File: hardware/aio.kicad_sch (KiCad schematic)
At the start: 48 parts, among them Q1 FCX690BTA, Q2 NTF2955T1G, Q3 MMBT2907ALT1G, U1 XTR117AIDGKR, U10 REF3040AIDBZR, U11 KF301-5.0-2P, U12 TLV9301IDBVR, U2 ISO7041FDBQR, U23 KF301-5.0-2P, U28 DAC8551IADGKR, U4 DAC60501MDGSR, U5 XTR111AIDGQR, U6 TLV9301IDBVR, U7 INA226AIDGSR, U8 DAC60501MDGSR, U9 DAC60501MDGSR

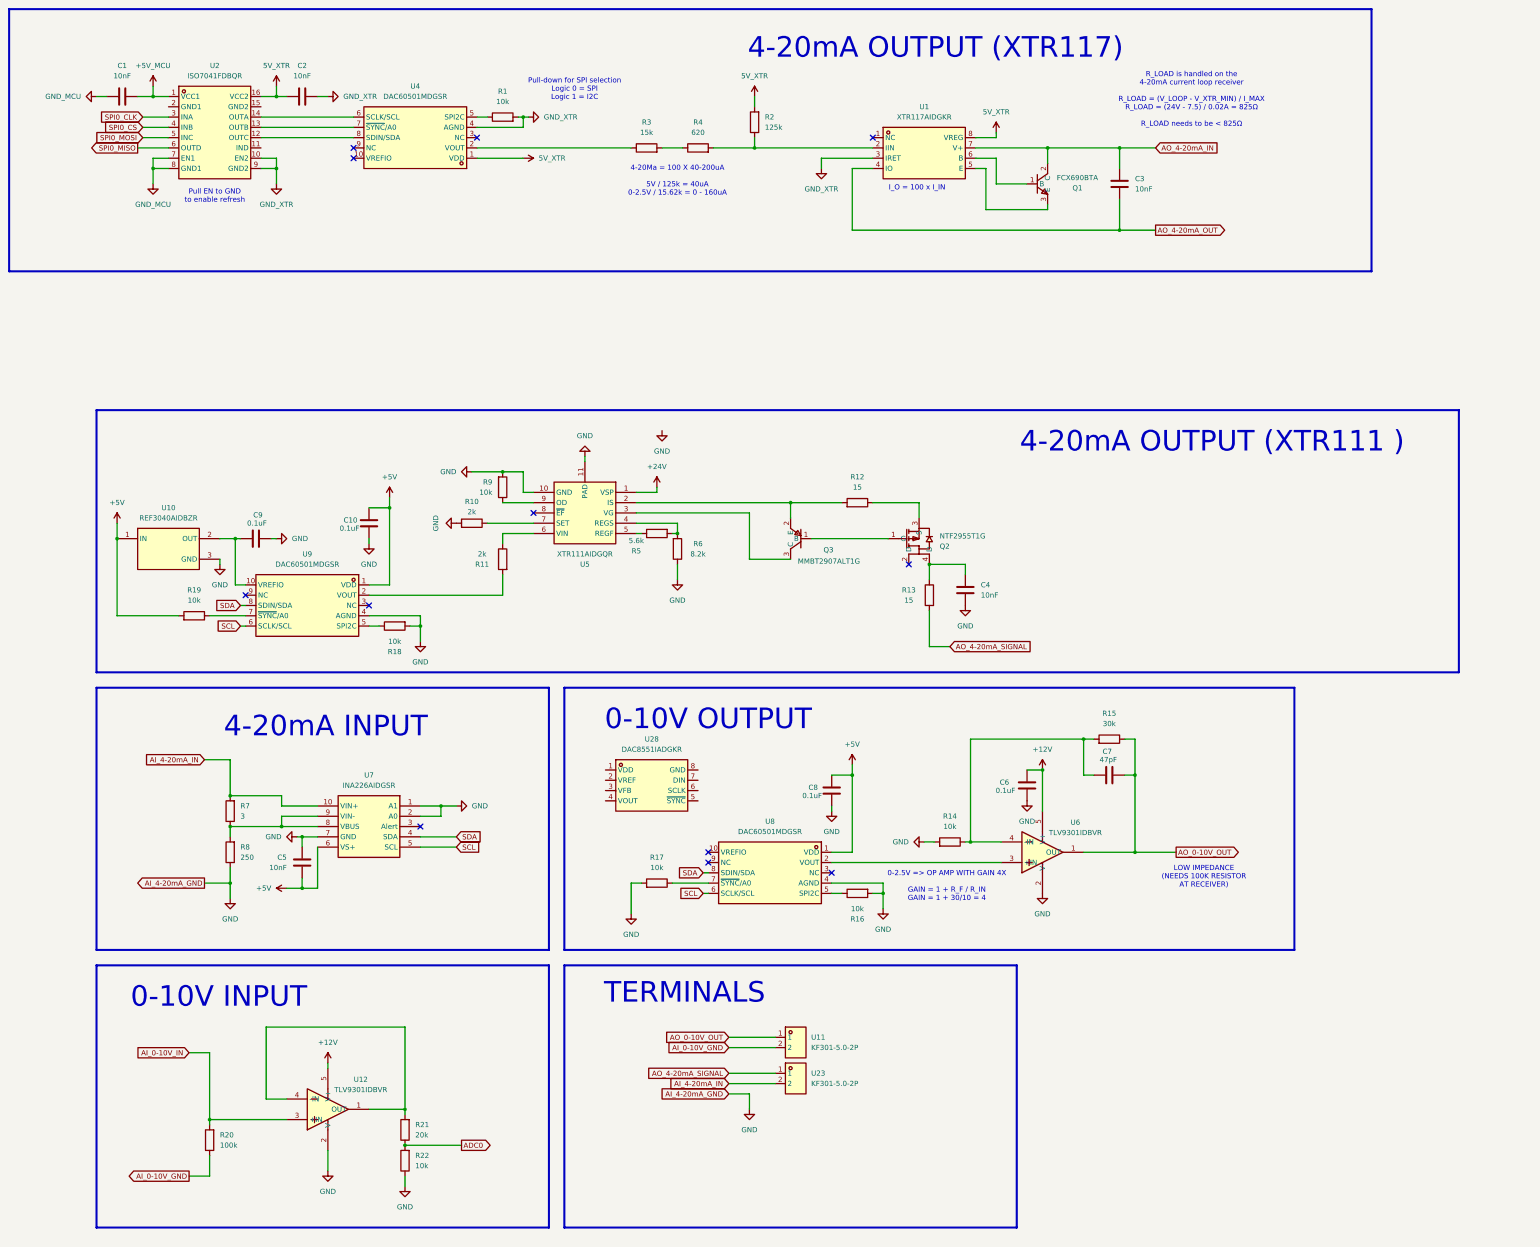
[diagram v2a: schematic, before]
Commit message: Board complete
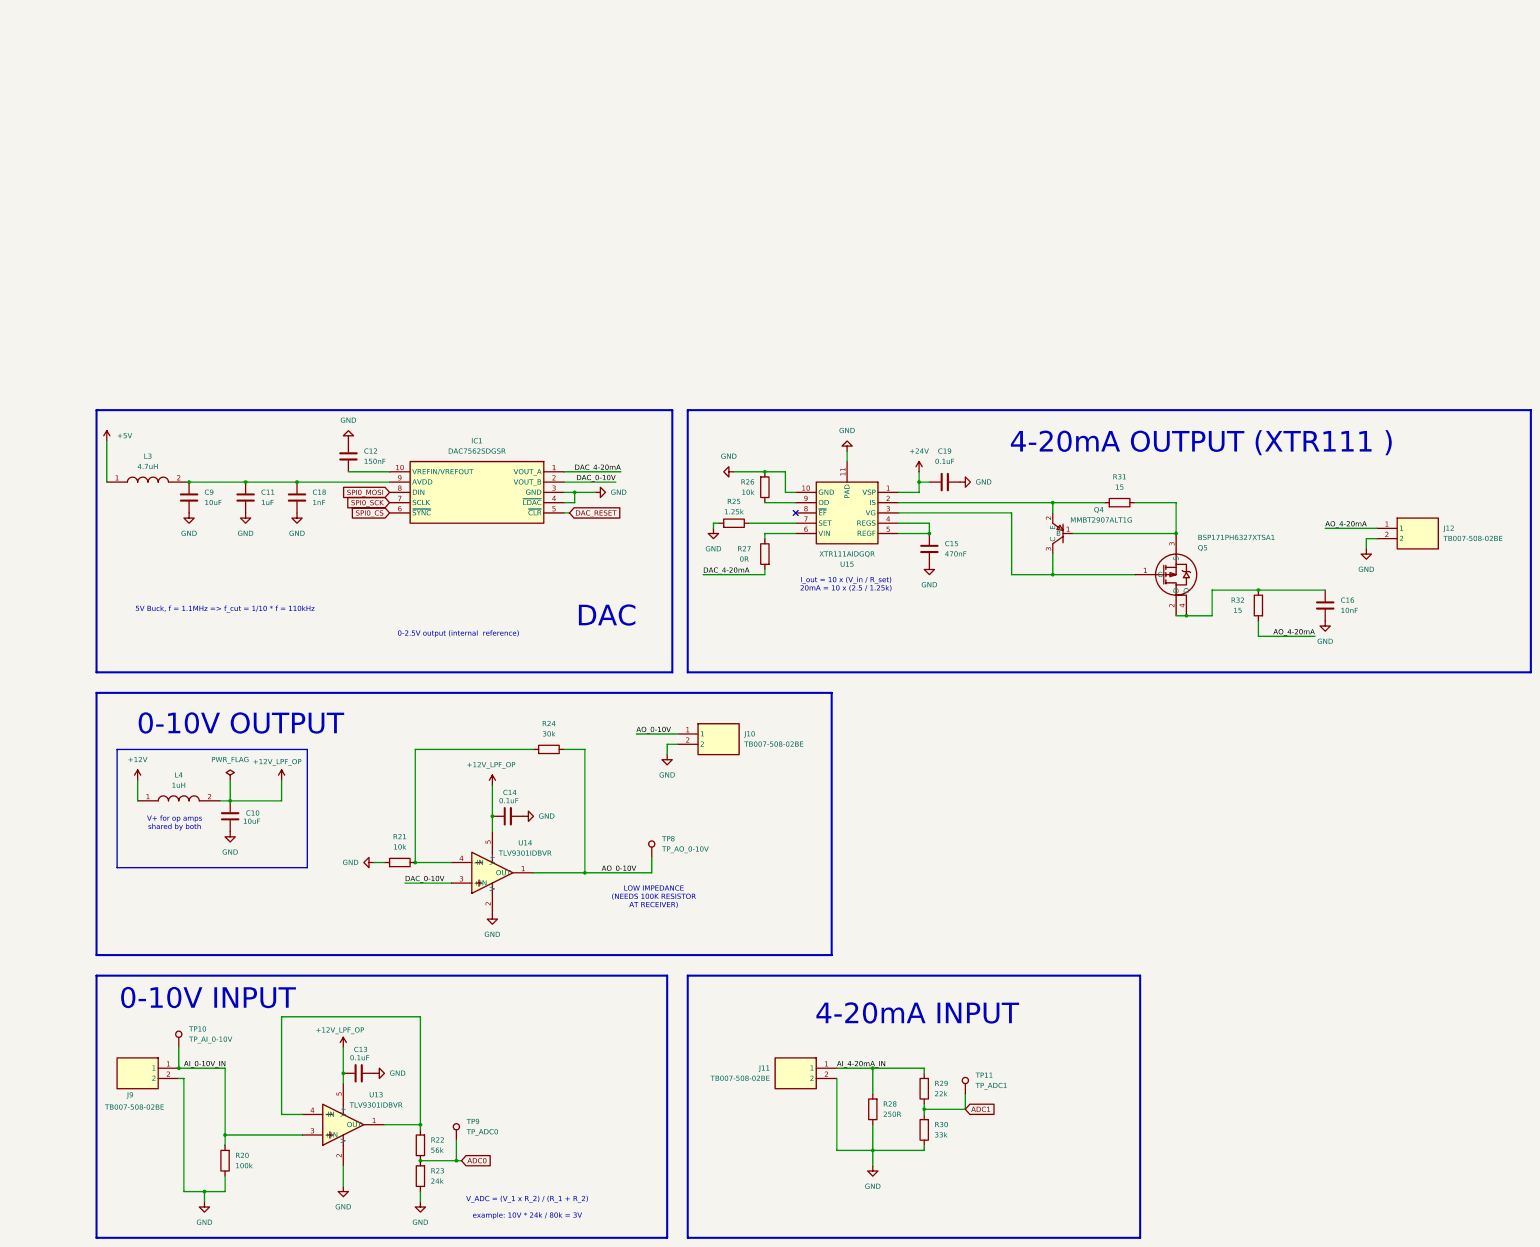
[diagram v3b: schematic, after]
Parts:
- removed C1, C2, C3, C5: 10nF, symbol Device:C
- removed C6, C8: 0.1uF, symbol Device:C
- removed C7: 47pF, symbol Device:C
- removed Q1: FCX690BTA, EasyEDA:SOT-89-3_L4.5-W2.5-P1.50-LS4.2-BR, symbol EasyEDA:FCX690BTA
- removed Q2: NTF2955T1G, EasyEDA:SOT-223-4_L6.5-W3.5-P2.30-LS7.0-BR, symbol EasyEDA:NTF2955T1G
- removed R1, R16, R17, R18, R19: 10k, symbol Device:R
- removed R2: 125k, symbol Device:R
- removed R3: 15k, symbol Device:R
- removed R4: 620, symbol Device:R
- removed R5: 5.6k, symbol Device:R
- removed R6: 8.2k, symbol Device:R
- removed R7: 3, symbol Device:R
- removed U1: XTR117AIDGKR, EasyEDA:VSSOP-8_L3.0-W3.0-P0.65-LS5.0-BL, symbol EasyEDA:XTR117AIDGKR
- removed U10: REF3040AIDBZR, EasyEDA:SOT-23-3_L2.9-W1.6-P1.90-LS2.8-BR, symbol EasyEDA:REF3040AIDBZR
- removed U11, U23: KF301-5.0-2P, EasyEDA:CONN-TH_P5.00_KF301-5.0-2P, symbol EasyEDA:KF301-5.0-2P
- removed U2: ISO7041FDBQR, EasyEDA:SSOP-16_L4.9-W3.9-P0.64-LS6.0-BL, symbol EasyEDA:ISO7041FDBQR
- removed U28: DAC8551IADGKR, EasyEDA:VSSOP-8_L3.0-W3.0-P0.65-LS5.0-BL, symbol EasyEDA:DAC8551IADGKR
- removed U4, U8, U9: DAC60501MDGSR, EasyEDA:VSSOP-10_L3.0-W3.0-P0.50-LS4.9-BL, symbol EasyEDA:DAC60501MDGSR
- removed U7: INA226AIDGSR, EasyEDA:MSOP-10_L3.0-W3.0-P0.50-LS5.0-BL, symbol EasyEDA:INA226AIDGSR
- added C11: 1uF, Capacitor_SMD:C_1206_3216Metric_Pad1.33x1.80mm_HandSolder, symbol Device:C
- added C12: 150nF, Capacitor_SMD:C_1206_3216Metric_Pad1.33x1.80mm_HandSolder, symbol Device:C
- added C13, C14, C19: 0.1uF, Capacitor_SMD:C_1206_3216Metric_Pad1.33x1.80mm_HandSolder, symbol Device:C
- added C15: 470nF, Capacitor_SMD:C_1206_3216Metric_Pad1.33x1.80mm_HandSolder, symbol Device:C
- added C18: 1nF, Capacitor_SMD:C_1206_3216Metric_Pad1.33x1.80mm_HandSolder, symbol Device:C
- added IC1: DAC7562SDGSR, Samacsys:SOP50P490X110-10N, symbol Samacsys:DAC7562SDGSR
- added J10, J11, J12, J9: TB007-508-02BE, Samacsys:TB00750802BE, symbol Samacsys:TB007-508-02BE
- added L3: 4.7uH, Samacsys:INDC3225X120N, symbol Samacsys:LQM31PN4R7M00L
- added L4: 1uH, Samacsys:LQM31PN1R0M00L, symbol Samacsys:LQM31PN1R0M00L
- added Q5: BSP171PH6327XTSA1, EasyEDA:SOT-223-4_L6.5-W3.5-P2.30-LS7.0-BR, symbol EasyEDA:BSP171PH6327XTSA1
- added R29: 22k, Resistor_SMD:R_1206_3216Metric_Pad1.30x1.75mm_HandSolder, symbol Device:R
- added R30: 33k, Resistor_SMD:R_1206_3216Metric_Pad1.30x1.75mm_HandSolder, symbol Device:R
- added TP10: TP_AI_0-10V, TestPoint:TestPoint_THTPad_2.0x2.0mm_Drill1.0mm, symbol Connector:TestPoint
- added TP11: TP_ADC1, TestPoint:TestPoint_THTPad_2.0x2.0mm_Drill1.0mm, symbol Connector:TestPoint
- added TP8: TP_AO_0-10V, TestPoint:TestPoint_THTPad_2.0x2.0mm_Drill1.0mm, symbol Connector:TestPoint
- added TP9: TP_ADC0, TestPoint:TestPoint_THTPad_2.0x2.0mm_Drill1.0mm, symbol Connector:TestPoint
- C10, C9: value 0.1uF -> 10uF; footprint (none) -> Capacitor_SMD:C_1206_3216Metric_Pad1.33x1.80mm_HandSolder
- C16: renamed from C4; footprint (none) -> Capacitor_SMD:C_1206_3216Metric_Pad1.33x1.80mm_HandSolder
- R20: footprint (none) -> Resistor_SMD:R_1206_3216Metric_Pad1.30x1.75mm_HandSolder
- R21: renamed from R14; footprint (none) -> Resistor_SMD:R_1206_3216Metric_Pad1.30x1.75mm_HandSolder
- R22: renamed from R21; value 20k -> 56k; footprint (none) -> Resistor_SMD:R_1206_3216Metric_Pad1.30x1.75mm_HandSolder
- R23: renamed from R22; value 10k -> 24k; footprint (none) -> Resistor_SMD:R_1206_3216Metric_Pad1.30x1.75mm_HandSolder
- R24: renamed from R15; footprint (none) -> Resistor_SMD:R_1206_3216Metric_Pad1.30x1.75mm_HandSolder
- R25: renamed from R10; value 2k -> 1.25k; footprint (none) -> Resistor_SMD:R_1206_3216Metric_Pad1.30x1.75mm_HandSolder
- R26: renamed from R9; footprint (none) -> Resistor_SMD:R_1206_3216Metric_Pad1.30x1.75mm_HandSolder
- R27: renamed from R11; value 2k -> 0R; footprint (none) -> Resistor_SMD:R_1206_3216Metric_Pad1.30x1.75mm_HandSolder
- R28: renamed from R8; value 250 -> 250R; footprint (none) -> Resistor_SMD:R_1206_3216Metric_Pad1.30x1.75mm_HandSolder
- R31: renamed from R12; footprint (none) -> Resistor_SMD:R_1206_3216Metric_Pad1.30x1.75mm_HandSolder
- R32: renamed from R13; footprint (none) -> Resistor_SMD:R_1206_3216Metric_Pad1.30x1.75mm_HandSolder
- renumbered Q3 to Q4, U12 to U13, U6 to U14, U5 to U15
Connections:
- net AI_0-10V_GND is gone; now on net GND: R20.1
- net +12V: now also L4.1; no longer U13.5 (V+), U14.5 (V+)
- net +24V: now also C19.2
- net +5V: now also L3.1; no longer C10.2
- net ADC0: now also TP9.1
- net AI_0-10V_IN: now also J9.1, TP10.1
- net AI_4-20mA_IN: now also R28.2, J11.1, R29.2
- net GND: now also C10.2, C11.1, C12.2, C13.2, C14.2, C15.1, C18.1, C19.1, IC1.3 (GND), IC1.4 (~{LDAC}), J10.2, J11.2, J12.2, J9.2, R30.1; no longer C10.1
- net SPI0_CS: now also IC1.6 (~{SYNC})
- net SPI0_MOSI: now also IC1.8 (DIN)
- net at Q4.1 (B): now also R31.1, Q5.3 (S)
- net at Q4.3 (C), U15.3 (VG): now also Q5.1 (G)
- net DAC_0-10V: now reaches U14.3 (+IN)
- net DAC_0-10V: now also IC1.2 (VOUT_B)
- net at U15.5 (REGF): now also U15.4 (REGS), C15.2
- net DAC_4-20mA: now reaches R27.2
- net DAC_4-20mA: now also IC1.1 (VOUT_A)
- net at C16.2, R32.1: now also Q5.2 (D), Q5.4 (D)
- net at C9.1: now also C11.2, C18.2, IC1.9 (AVDD), L3.2
- net AO_0-10V_OUT renamed AO_0-10V
- net AO_0-10V: now also J10.1, TP8.1
- net AO_4-20mA_SIGNAL renamed AO_4-20mA
- net AO_4-20mA: now also J12.1
- new net: C12.1, IC1.10 (VREFIN/VREFOUT)
- new net +12V_LPF_OP: C10.1, C13.1, C14.1, L4.2, U13.5 (V+), U14.5 (V+)
- new net ADC1: R29.1, R30.2, TP11.1
- new net DAC_RESET: IC1.5 (~{CLR})
- new net SPI0_SCK: IC1.7 (SCLK)
- no-connect marks 12 -> 1
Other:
- note added: "0-2.5V output (internal reference)"
- note added: "5V Buck, f = 1.1MHz => f_cut = 1/10 * f = 110kHz"
- note added: "DAC"
- note added: "I_out = 10 x (V_in / R_set) 20mA = 10 x (2.5 / 1.25k)"
- note added: "V+ for op amps shared by both"
- note added: "V_ADC = (V_1 x R_2) / (R_1 + R_2) example: 10V * 24k / 80k = 3V"
- note removed: "0-2.5V => OP AMP WITH GAIN 4X GAIN = 1 + R_F / R_IN GAIN = 1 + 30/10 = 4"
- note removed: "4-20Ma = 100 X 40-200uA 5V / 125k = 40uA 0-2.5V / 15.62k = 0 - 160uA"
- note removed: "4-20mA OUTPUT (XTR117)"
- note removed: "I_O = 100 x I_IN"
- note removed: "Pull EN to GND to enable refresh"
- note removed: "Pull-down for SPI selection Logic 0 = SPI Logic 1 = I2C"
- note removed: "R_LOAD is handled on the 4-20mA current loop receiver R_LOAD = (V_LOOP - V_XTR_MIN) / I_MAX R_LOAD = (24V - 7.5) / 0.02A = 825Ω R_LOAD needs to be < 825Ω"
- note removed: "TERMINALS"
- moved on the sheet: C16, Q4, R20, R21, R22, R23, R24, R25, R26, R27, R28, R31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
